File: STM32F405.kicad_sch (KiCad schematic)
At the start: 25 parts, among them SW1 SW_MEC_5G, SW2 SW_DIP_x04, U3 STM32F405RGTx, Y1 25MHz

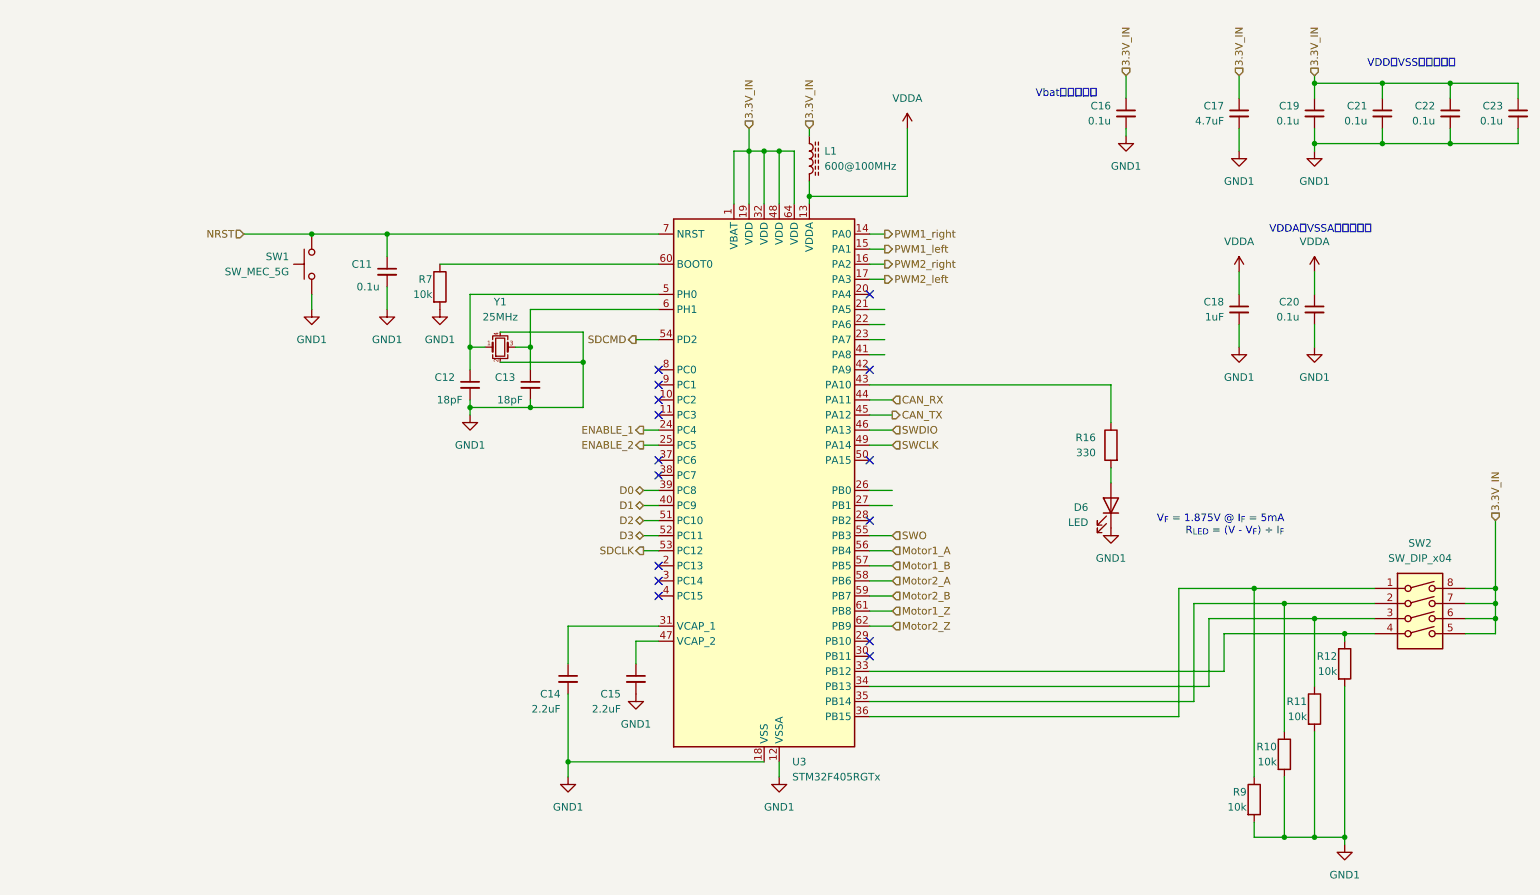
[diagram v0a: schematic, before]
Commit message: 制御回路完成
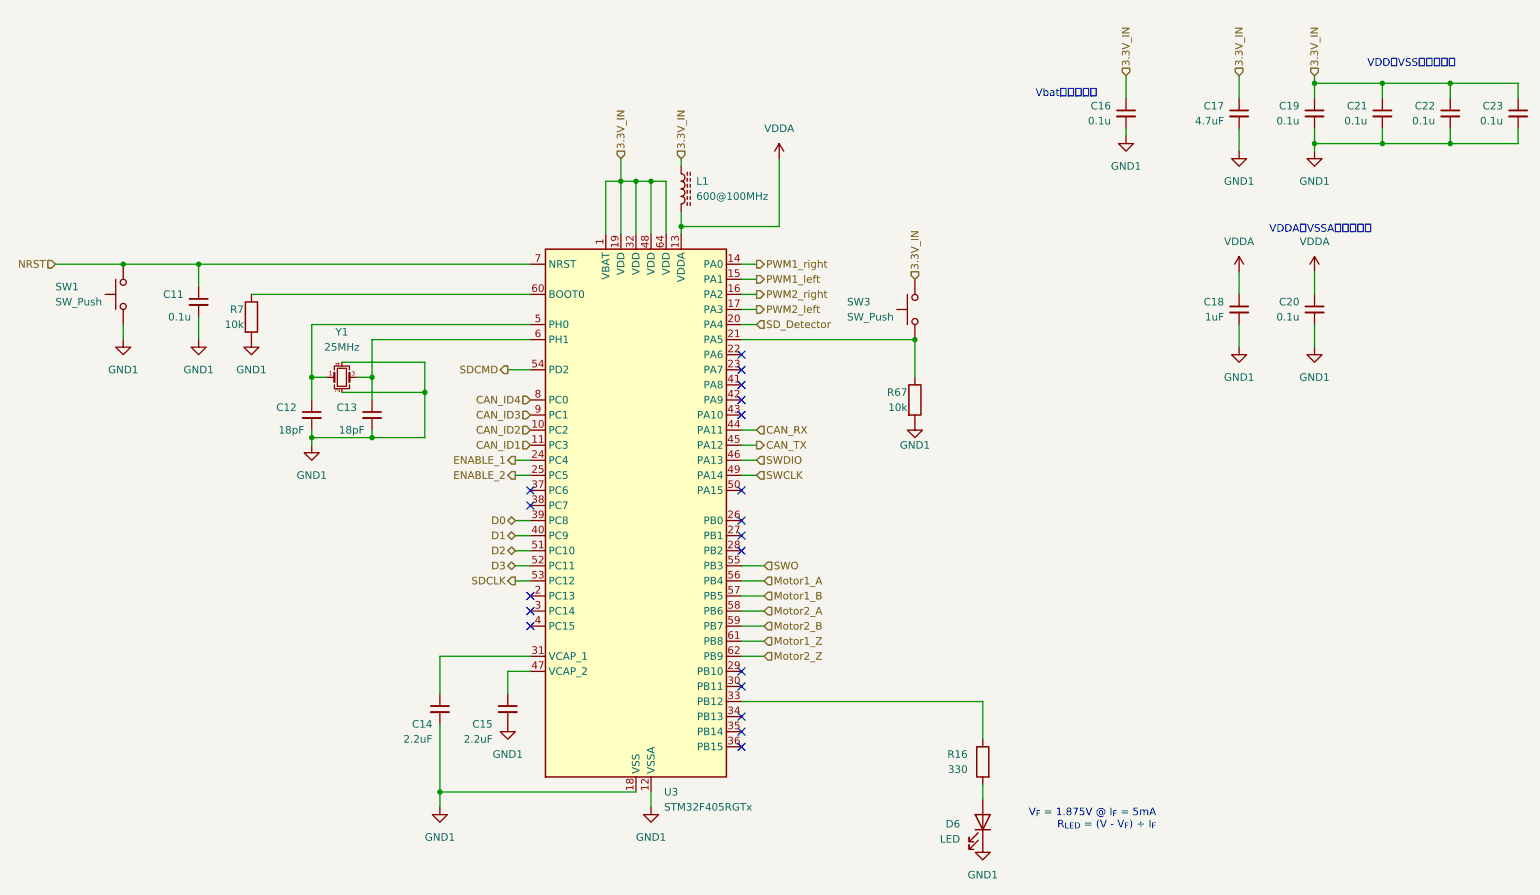
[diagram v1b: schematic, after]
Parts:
- removed R10, R11, R12, R9: 10k, Resistor_SMD:R_0402_1005Metric, symbol Device:R
- removed SW1: SW_MEC_5G, RDC_footprint:TVBP06-B043, symbol Switch:SW_MEC_5G
- removed SW2: SW_DIP_x04, Button_Switch_SMD:SW_DIP_SPSTx04_Slide_Copal_CHS-04B_W7.62mm_P1.27mm, symbol Switch:SW_DIP_x04
- added R67: 10k, Resistor_SMD:R_0402_1005Metric, symbol Device:R
- added SW1, SW3: SW_Push, RDC_footprint:TVBP06-B043, symbol Switch:SW_Push
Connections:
- net 3.3V_IN: now also SW3.2
- net GND1: now also R67.2, SW1.1
- net NRST: now also SW1.2
- net at R16.1: now also U3.33 (PB12); no longer U3.43 (PA10)
- net CAN_ID2: now reaches U3.10 (PC2)
- net CAN_ID1: now reaches U3.11 (PC3)
- net SD_Detector: now reaches U3.20 (PA4)
- net at U3.21 (PA5): now also R67.1, SW3.1
- net CAN_ID4: now reaches U3.8 (PC0)
- net CAN_ID3: now reaches U3.9 (PC1)
- no-connect marks 15 -> 19
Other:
- moved on the sheet: C11, C12, C13, C14, C15, L1, R7, U3, Y1
